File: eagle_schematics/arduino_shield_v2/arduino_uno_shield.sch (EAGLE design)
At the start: 16 parts, among them IC1 TL072P

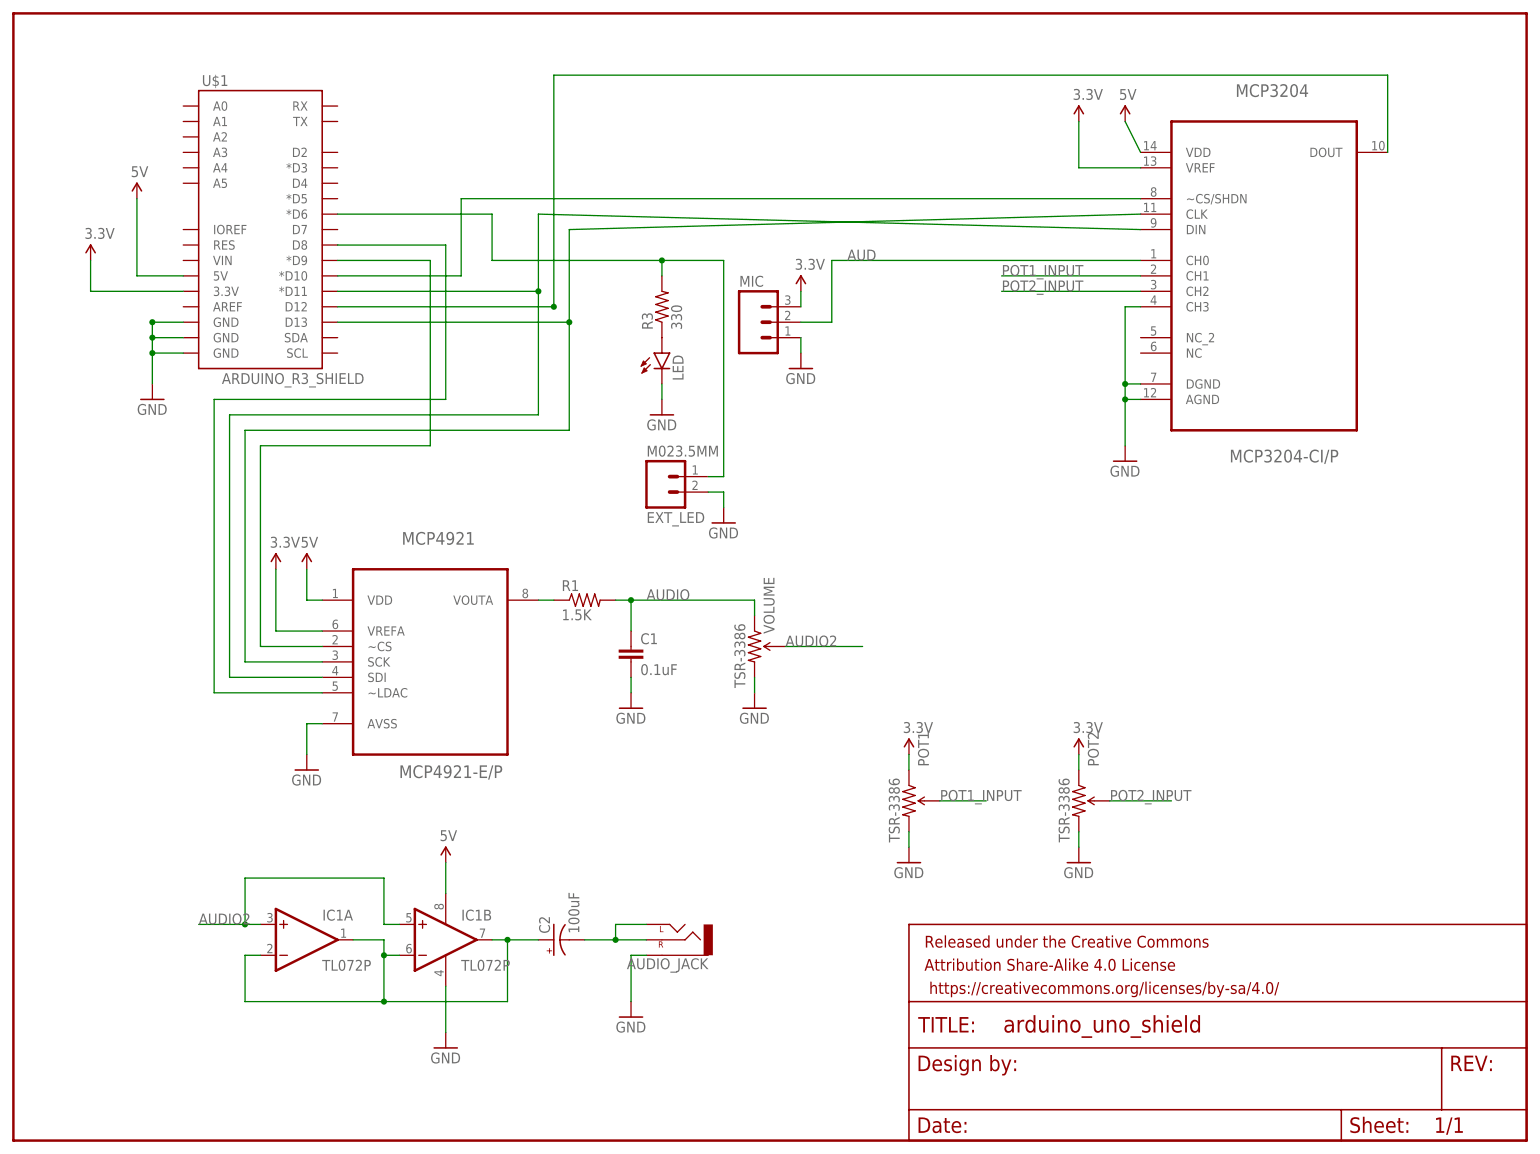
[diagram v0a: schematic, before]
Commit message: refine board layout
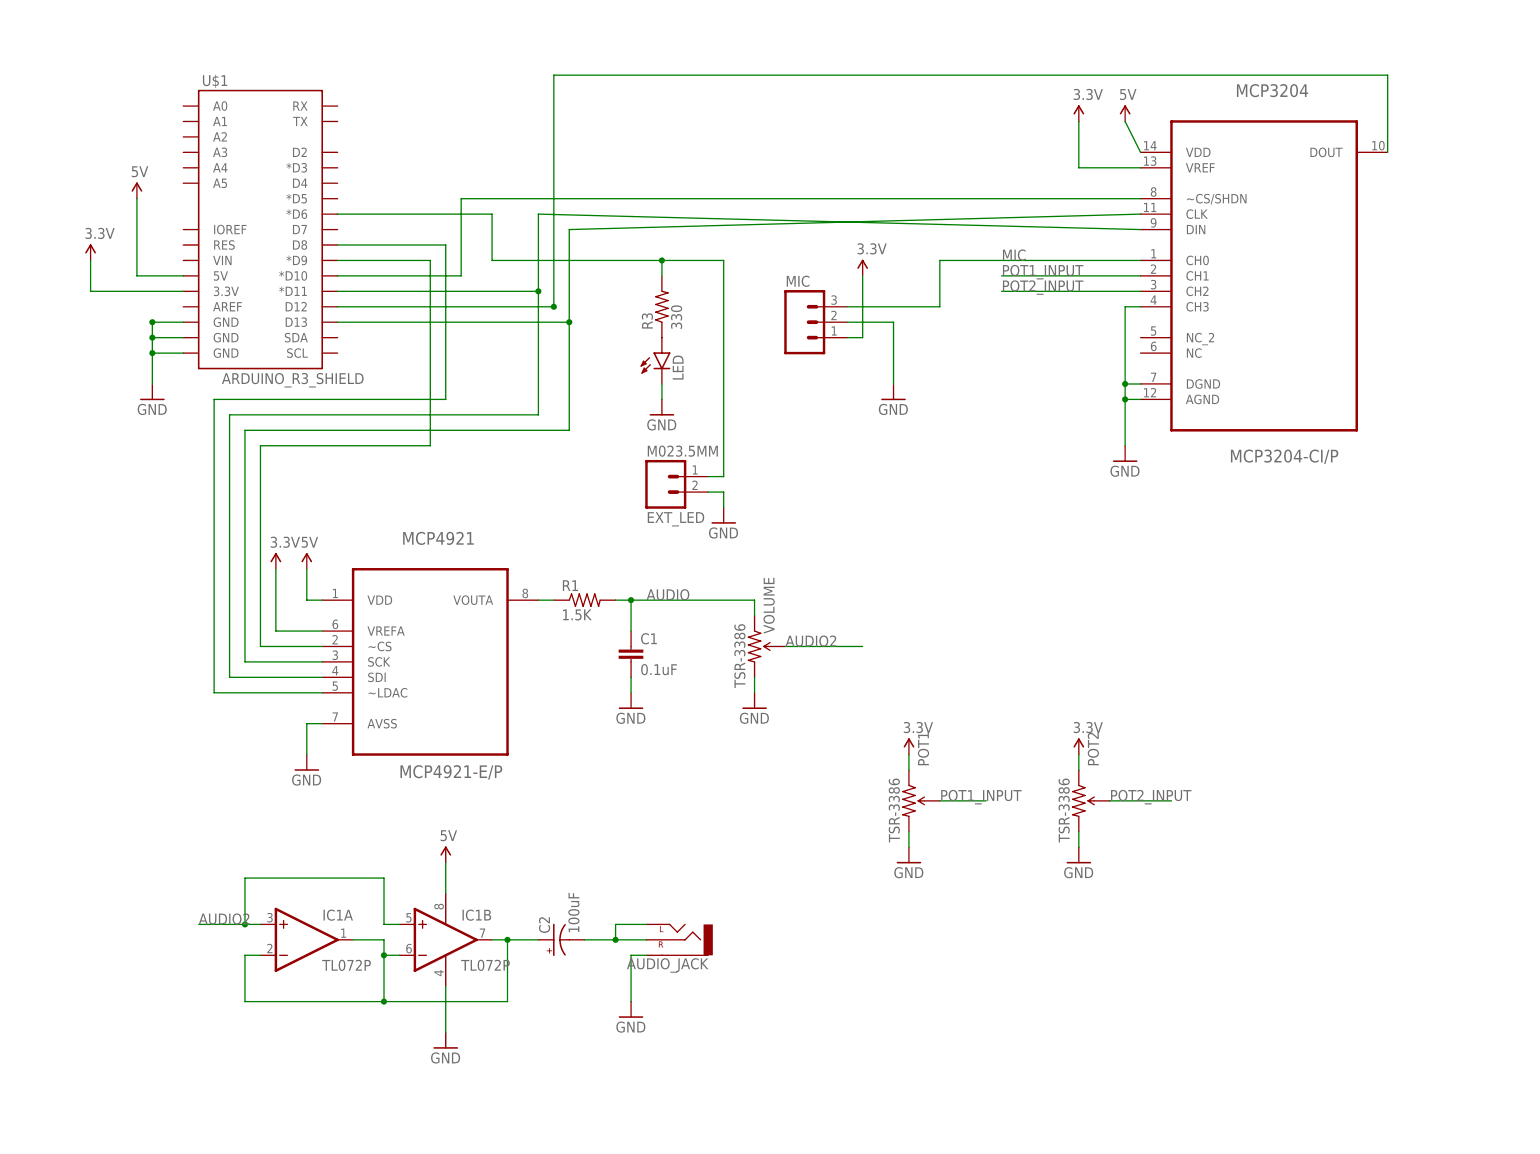
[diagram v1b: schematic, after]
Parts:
- removed FRAME3: FRAME-LETTER, SparkFun-Aesthetics:FRAME-LETTER
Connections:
- removed net AUD: MCP3204.CH0, MIC.2
- new net MIC: MCP3204.CH0, MIC.3
- net 3.3V: now also MIC.1; no longer MIC.3
- net GND: now also MIC.2; no longer MIC.1
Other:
- moved on the sheet: MIC
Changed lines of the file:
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@@
 <part name="GND14" library="SparkFun-Aesthetics" deviceset="GND" device=""/>
 <part name="EXT_LED" library="SparkFun-Connectors" deviceset="M02" device="3.5MM"/>
-<part name="FRAME3" library="SparkFun-Aesthetics" deviceset="FRAME-LETTER" device=""/>
 <part name="IC1" library="linear" deviceset="TL072" device="P"/>
 <part name="SUPPLY15" library="SparkFun-Aesthetics" deviceset="5V" device=""/>
@@
 <instance part="GND1" gate="1" x="-68.58" y="-7.62"/>
 <instance part="AUDIO_JACK" gate="G$1" x="-60.96" y="-45.72" rot="R180"/>
-<instance part="MIC" gate="G$1" x="-48.26" y="55.88" smashed="yes">
-<attribute name="VALUE" x="-50.8" y="48.26" size="1.778" layer="96"/>
-<attribute name="NAME" x="-50.8" y="61.722" size="1.778" layer="95"/>
+<instance part="MIC" gate="G$1" x="-40.64" y="55.88" smashed="yes">
+<attribute name="VALUE" x="-43.18" y="48.26" size="1.778" layer="96"/>
+<attribute name="NAME" x="-43.18" y="61.722" size="1.778" layer="95"/>
 </instance>
 <instance part="LED" gate="G$1" x="-63.5" y="50.8"/>
@@
 <instance part="SUPPLY5" gate="G$1" x="-127" y="15.24"/>
 <instance part="SUPPLY6" gate="G$1" x="5.08" y="88.9"/>
-<instance part="SUPPLY7" gate="G$1" x="-40.64" y="60.96"/>
-<instance part="GND4" gate="1" x="-40.64" y="48.26"/>
+<instance part="SUPPLY7" gate="G$1" x="-30.48" y="63.5"/>
+<instance part="GND4" gate="1" x="-25.4" y="43.18"/>
 <instance part="SUPPLY8" gate="G$1" x="-22.86" y="-15.24"/>
 <instance part="GND5" gate="1" x="-22.86" y="-33.02"/>
@@
 <instance part="GND14" gate="1" x="-53.34" y="22.86"/>
 <instance part="EXT_LED" gate="G$1" x="-63.5" y="30.48" rot="MR180"/>
-<instance part="FRAME3" gate="G$1" x="-170.18" y="-78.74"/>
-<instance part="FRAME3" gate="G$2" x="-22.86" y="-78.74"/>
 <instance part="IC1" gate="A" x="-121.92" y="-45.72"/>
 <instance part="IC1" gate="B" x="-99.06" y="-45.72"/>
@@
 </segment>
 <segment>
-<pinref part="MIC" gate="G$1" pin="1"/>
-<pinref part="GND4" gate="1" pin="GND"/>
-<wire x1="-40.64" y1="50.8" x2="-40.64" y2="53.34" width="0.1524" layer="91"/>
-</segment>
-<segment>
 <pinref part="MCP4921" gate="A" pin="AVSS"/>
 <pinref part="GND8" gate="1" pin="GND"/>
@@
 <wire x1="12.7" y1="58.42" x2="15.24" y2="58.42" width="0.1524" layer="91"/>
 </segment>
+<segment>
+<pinref part="MIC" gate="G$1" pin="2"/>
+<wire x1="-33.02" y1="55.88" x2="-25.4" y2="55.88" width="0.1524" layer="91"/>
+<pinref part="GND4" gate="1" pin="GND"/>
+<wire x1="-25.4" y1="55.88" x2="-25.4" y2="45.72" width="0.1524" layer="91"/>
+</segment>
 </net>
 <net name="5V" class="0">
@@
 </segment>
 <segment>
-<pinref part="MIC" gate="G$1" pin="3"/>
-<pinref part="SUPPLY7" gate="G$1" pin="3.3V"/>
-<wire x1="-40.64" y1="58.42" x2="-40.64" y2="60.96" width="0.1524" layer="91"/>
-</segment>
-<segment>
 <pinref part="SUPPLY1" gate="G$1" pin="3.3V"/>
 <wire x1="-157.48" y1="66.04" x2="-157.48" y2="60.96" width="0.1524" layer="91"/>
@@
 <pinref part="POT2" gate="R?" pin="CCW"/>
 <wire x1="5.08" y1="-15.24" x2="5.08" y2="-17.78" width="0.1524" layer="91"/>
+</segment>
+<segment>
+<pinref part="MIC" gate="G$1" pin="1"/>
+<wire x1="-33.02" y1="53.34" x2="-30.48" y2="53.34" width="0.1524" layer="91"/>
+<pinref part="SUPPLY7" gate="G$1" pin="3.3V"/>
+<wire x1="-30.48" y1="53.34" x2="-30.48" y2="63.5" width="0.1524" layer="91"/>
 </segment>
 </net>
@@
 <wire x1="-132.08" y1="38.1" x2="-78.74" y2="38.1" width="0.1524" layer="91"/>
 <wire x1="-78.74" y1="38.1" x2="-78.74" y2="55.88" width="0.1524" layer="91"/>
-</segment>
-</net>
-<net name="AUD" class="0">
-<segment>
-<pinref part="MIC" gate="G$1" pin="2"/>
-<wire x1="-40.64" y1="55.88" x2="-35.56" y2="55.88" width="0.1524" layer="91"/>
-<wire x1="-35.56" y1="55.88" x2="-35.56" y2="66.04" width="0.1524" layer="91"/>
-<pinref part="MCP3204" gate="A" pin="CH0"/>
-<wire x1="-35.56" y1="66.04" x2="15.24" y2="66.04" width="0.1524" layer="91"/>
-<label x="-33.02" y="66.04" size="1.778" layer="95"/>
 </segment>
 </net>
@@
 </segment>
 </net>
+<net name="MIC" class="0">
+<segment>
+<pinref part="MIC" gate="G$1" pin="3"/>
+<wire x1="-33.02" y1="58.42" x2="-17.78" y2="58.42" width="0.1524" layer="91"/>
+<wire x1="-17.78" y1="58.42" x2="-17.78" y2="66.04" width="0.1524" layer="91"/>
+<pinref part="MCP3204" gate="A" pin="CH0"/>
+<wire x1="-17.78" y1="66.04" x2="15.24" y2="66.04" width="0.1524" layer="91"/>
+<label x="-7.62" y="66.04" size="1.778" layer="95"/>
+</segment>
+</net>
